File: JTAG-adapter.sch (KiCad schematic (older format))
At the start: 6 parts

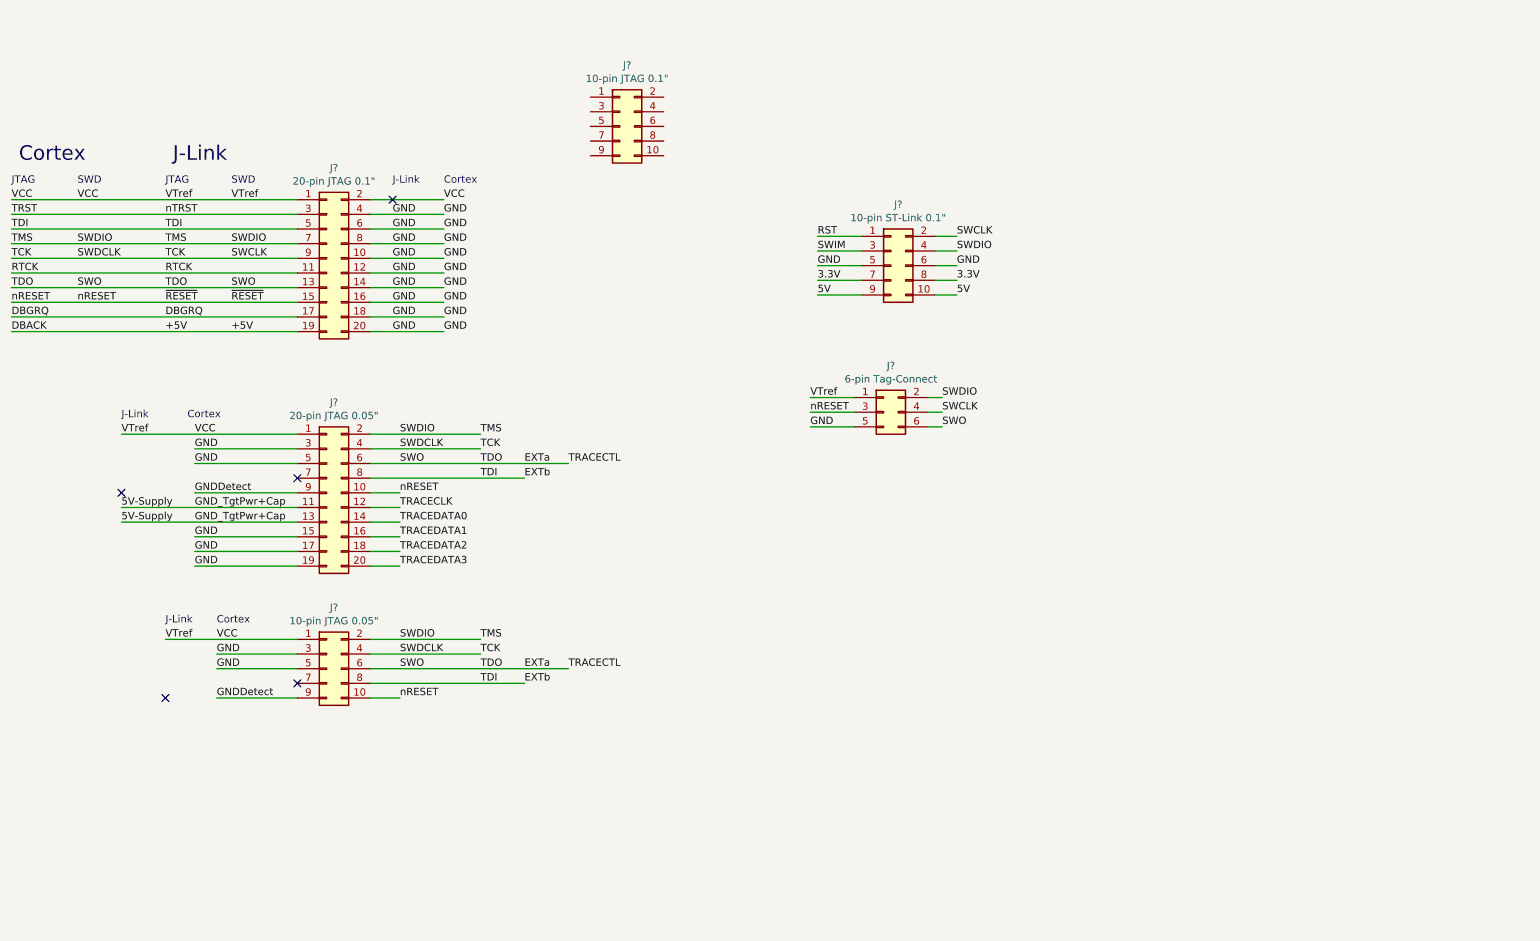
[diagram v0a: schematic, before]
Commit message: Draft of schematic and layout
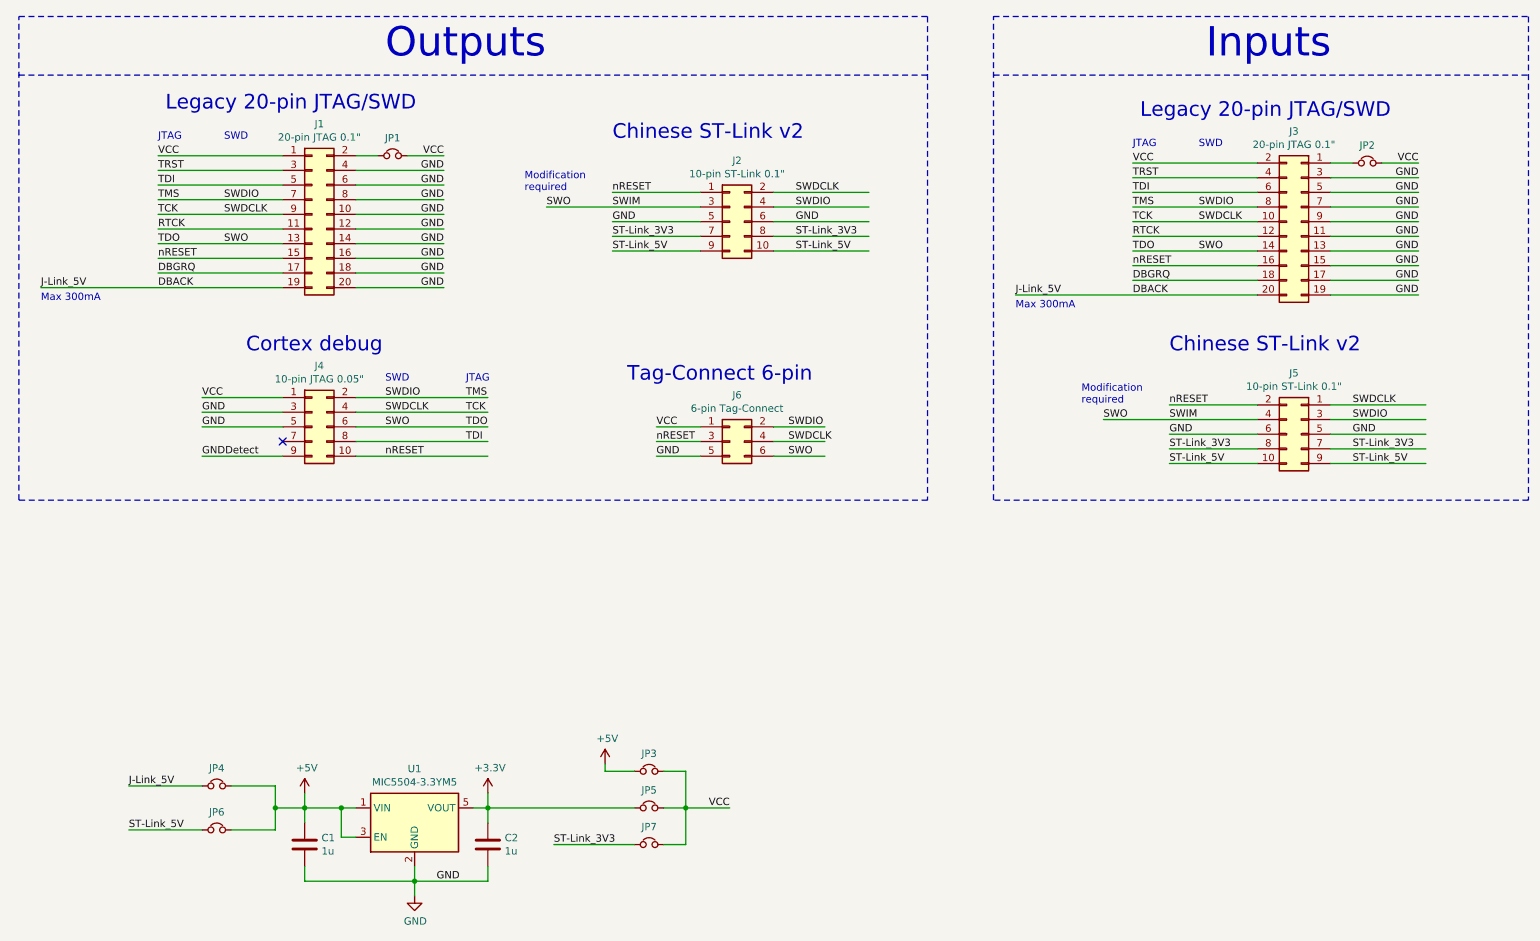
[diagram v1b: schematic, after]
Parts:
- removed J?: 10-pin JTAG 0.1\", symbol Connector_Generic:Conn_02x05_Odd_Even
- removed J?: 20-pin JTAG 0.05\", symbol Connector_Generic:Conn_02x10_Odd_Even
- added C1, C2: 1u, Capacitor_SMD:C_0603_1608Metric, symbol Device:C
- added J3: 20-pin JTAG 0.1\", Connector_PinSocket_2.54mm:PinSocket_2x10_P2.54mm_Horizontal, symbol Connector_Generic:Conn_02x10_Odd_Even
- added J5: 10-pin ST-Link 0.1\", Connector_PinSocket_2.54mm:PinSocket_2x05_P2.54mm_Horizontal, symbol Connector_Generic:Conn_02x05_Odd_Even
- added JP1, JP2, JP3, JP4, JP5, JP6, JP7: ~, Connector_PinHeader_2.54mm:PinHeader_1x02_P2.54mm_Vertical, symbol Device:Jumper_NC_Small
- added U1: MIC5504-3.3YM5, Package_TO_SOT_SMD:SOT-23-5, symbol Regulator_Linear:MIC5504-3.3YM5
- J1: renamed from J?; footprint (none) -> Connector_IDC:IDC-Header_2x10_P2.54mm_Vertical
- J2: renamed from J?; footprint (none) -> Connector_IDC:IDC-Header_2x05_P2.54mm_Vertical
- J4: renamed from J?; footprint (none) -> Connector_PinHeader_1.27mm:PinHeader_2x05_P1.27mm_Vertical
- J6: renamed from J?; footprint (none) -> Connector_IDC:IDC-Header_2x03_P2.54mm_Vertical
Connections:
- net labels added: +3.3V, J-Link_5V, ST-Link_3V3, ST-Link_5V
- net labels removed: 3.3V, 5V, 5V-Supply, EXTa, EXTb, GND_TgtPwr+Cap, RST, SWCLK, TRACECLK, TRACECTL, TRACEDATA0, TRACEDATA1, TRACEDATA2, TRACEDATA3, VTref, nTRST, ~RESET
- wire segments 64 -> 109
- no-connect marks 5 -> 1
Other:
- note added: "Chinese ST-Link v2"
- note added: "Cortex debug"
- note added: "Inputs"
- note added: "Legacy 20-pin JTAG/SWD"
- note added: "Max 300mA"
- note added: "Modification\nrequired"
- note added: "Outputs"
- note added: "Tag-Connect 6-pin"
- note removed: "Cortex"
- note removed: "J-Link"
- moved on the sheet: J1, J2, J4, J6
